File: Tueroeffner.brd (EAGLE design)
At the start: 54.6 x 22.9 mm, 34 parts, among them IC1 NCP1117ST33T3G, IC3 M25PE20, K2 EC2-12TNU, Q1 2N7002CK, Q2 2N7002CK

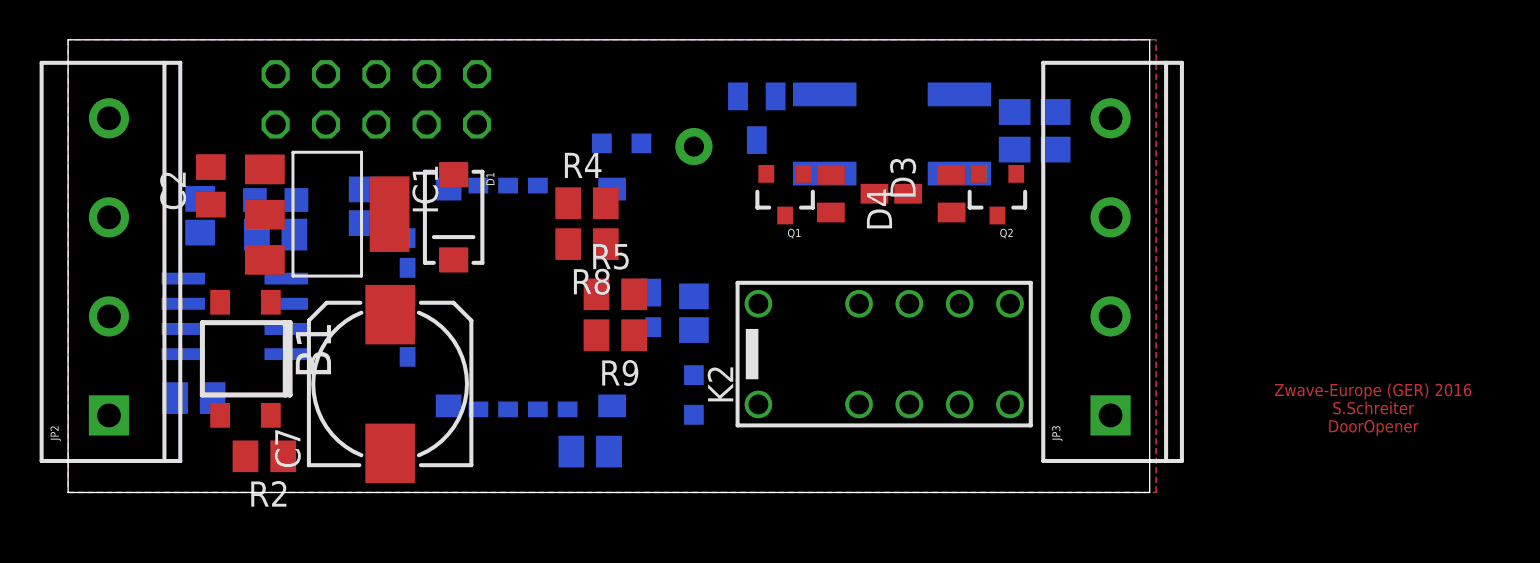
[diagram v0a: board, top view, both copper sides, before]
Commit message: Semi Routed
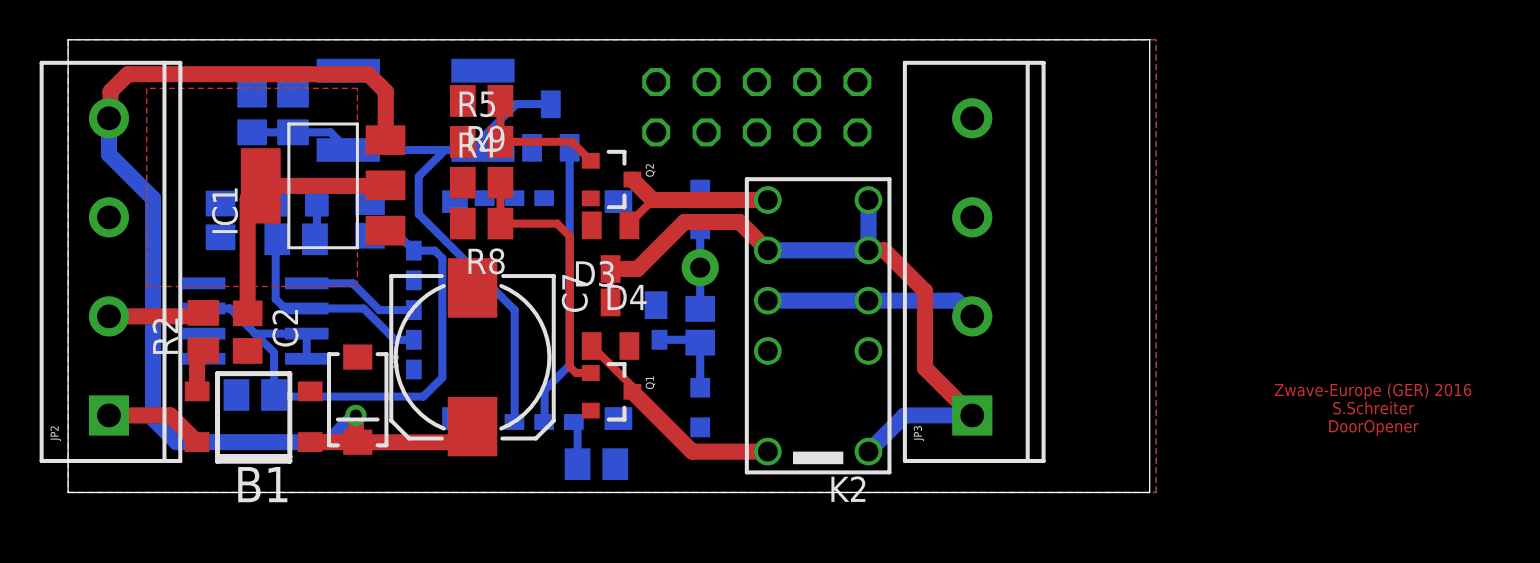
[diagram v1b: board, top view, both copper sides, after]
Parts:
- C7: value 470µF 16V -> 470µF 25V
- moved C5 40.6 mm to (7.70, 17.9), turned to 90 degrees
- moved R1 36.4 mm to (9.76, 17.9), turned to 90 degrees
- moved U$1 24.1 mm to (16.0, 18.0), turned to 0 degrees
- moved Q2 19.5 mm to (25.8, 14.5), turned to 270 degrees
- moved SV3 19.2 mm to (33.2, 18.2), turned to 0 degrees
- moved D4 16.3 mm to (25.8, 11.1), turned to 180 degrees
- moved D3 13.9 mm to (25.8, 7.22), turned to 0 degrees
- moved R9 13.6 mm to (19.3, 18.5)
- moved Q1 13.3 mm to (25.8, 3.81), turned to 270 degrees
- moved D2 10.4 mm to (22.8, 17.2), turned to 0 degrees
- moved D1 10.4 mm to (13.0, 3.41)
- moved R5 10.2 mm to (19.3, 16.4)
- moved C2 7.61 mm to (7.48, 6.83), turned to 270 degrees
- moved R2 7.00 mm to (5.24, 6.84), turned to 90 degrees
- moved JP3 6.98 mm to (44.1, 2.62)
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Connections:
- net AC_5-12V1: now also B1.AC1; no longer B1.AC2
- net N$1: now also B1.AC2; no longer B1.AC1
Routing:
- net DC_5-12V: track 0.00 -> 91.5 mm, vias 0 -> 1
- net VCC-3.3V: track 0.00 -> 42.6 mm
- net BUTTON: track 0.00 -> 35.0 mm
- net INT1: track 0.00 -> 14.4 mm
- net RELAY0: track 0.00 -> 13.6 mm
- net N$6: track 0.00 -> 11.2 mm
- net SCK: track 0.00 -> 10.9 mm
- net RELAY: track 0.00 -> 10.6 mm
- net N$7: track 0.00 -> 9.04 mm
- net RELAY1: track 0.00 -> 7.02 mm
- net MOSI: track 0.00 -> 5.97 mm
- net AC_5-12V1: track 0.00 -> 5.00 mm
- net AC_5-12V0: track 0.00 -> 4.83 mm
- net ANTENNA: track 0.00 -> 4.39 mm
- net N$33: track 0.00 -> 4.02 mm
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- added copper zone on layer 1, net VCC-3.3V

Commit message: Auto Router
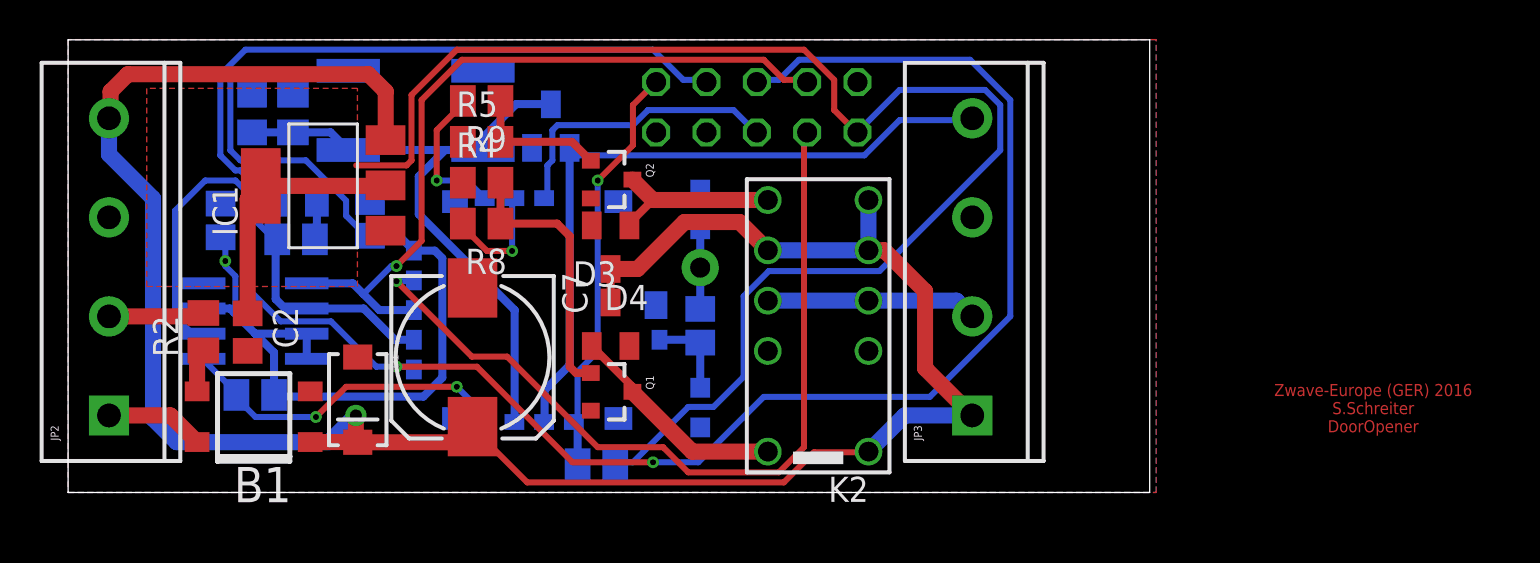
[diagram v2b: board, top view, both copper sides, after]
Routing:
- net VCC-3.3V: track 42.6 -> 134.6 mm, vias 0 -> 1
- net MISO: track 0.00 -> 87.7 mm, vias 0 -> 2
- net RXD: track 0.00 -> 41.9 mm, vias 0 -> 1
- net SCK: track 10.9 -> 46.4 mm
- net MOSI: track 5.97 -> 37.9 mm, vias 0 -> 1
- net DC_5-12V: track 91.5 -> 113.3 mm
- net INT1: track 14.4 -> 35.7 mm
- net RESET: track 2.21 -> 21.1 mm, vias 0 -> 1
- net CS: track 0.00 -> 17.2 mm, vias 0 -> 2
- net TXD: track 0.00 -> 14.8 mm
- net N$5: track 0.00 -> 7.34 mm, vias 0 -> 1
- net N$4: track 0.00 -> 5.90 mm, vias 0 -> 1
